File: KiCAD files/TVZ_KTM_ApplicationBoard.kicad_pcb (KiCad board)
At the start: 2 copper layers, 146 x 55 mm, 114 parts, among them J1 Conn_02x19_Odd_Even, J2 Conn_02x19_Odd_Even, J3 Conn_02x19_Odd_Even, J4 Conn_02x19_Odd_Even, SW1 EG1271A, SW2 EG1271A, SW3 EG1271A, SW4 EG1271A, U1 LM75B, U2 MCP2551-I-P, U3 MCP2551-I-P

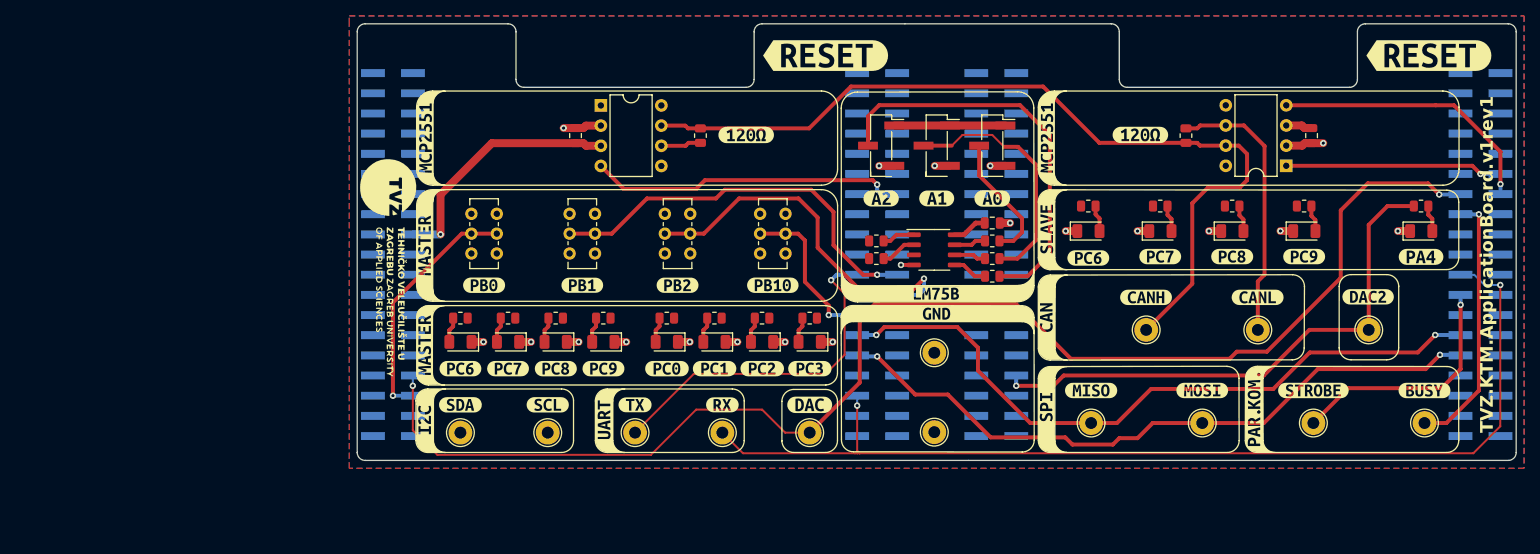
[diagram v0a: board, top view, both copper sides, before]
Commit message: update
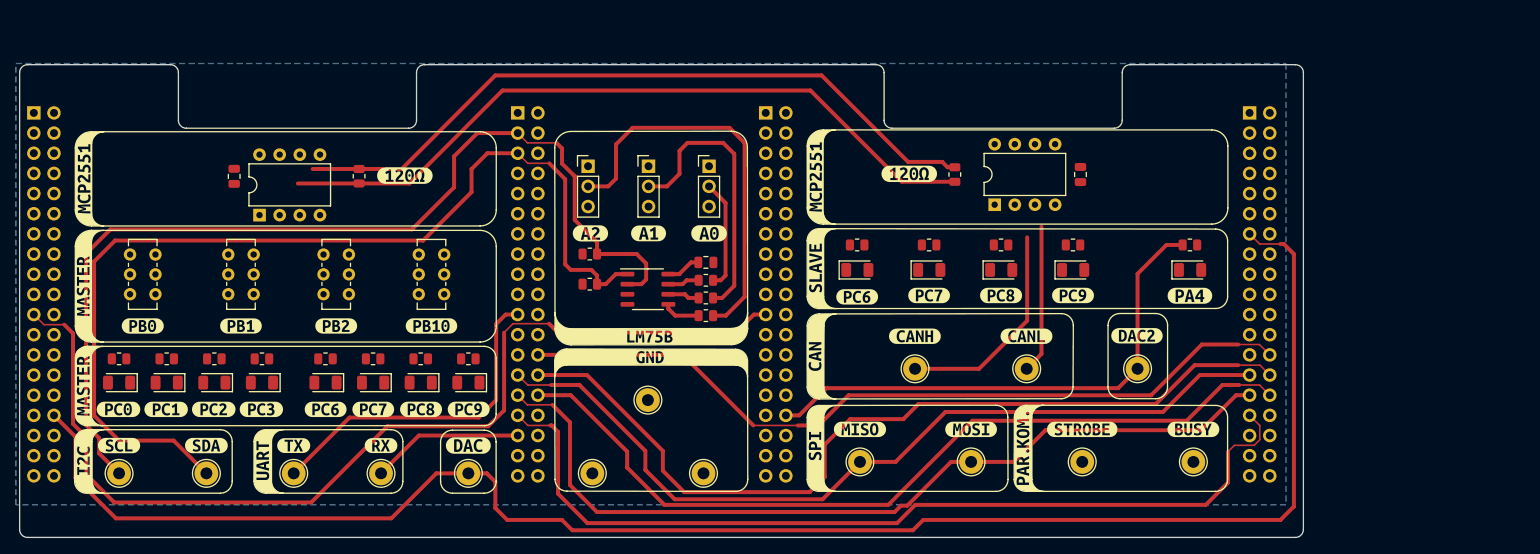
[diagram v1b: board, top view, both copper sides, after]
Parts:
- removed G***: LOGO, Footprint:tvz3
- removed kibuzzard-63D0F0B6 (x2): G***, kibuzzard-63D0F0B6
- added TP15: TestPoint, Footprint:KEYS4952, F.Cu at (143.6, 106.6)
- J1, J2, J3, J4: footprint Connector_PinSocket_2.54mm:PinSocket_2x19_P2.54mm_Vertical_SMD -> Connector_PinSocket_2.54mm:PinSocket_2x19_P2.54mm_Vertical
- JP1, JP4, JP5: footprint Connector_PinHeader_2.54mm:PinHeader_1x03_P2.54mm_Vertical_SMD_Pin1Right -> Connector_PinHeader_2.54mm:PinHeader_1x03_P2.54mm_Vertical
- moved kibuzzard-64A69B51 69.3 mm to (69.9, 98.6)
- moved kibuzzard-64A69B71 69.3 mm to (75.9, 98.6)
- moved kibuzzard-64A69B81 69.3 mm to (81.9, 98.6)
- moved kibuzzard-64A69B8B 69.3 mm to (87.9, 98.6)
- moved TP6 54.2 mm to (70.0, 106.6)
- moved kibuzzard-63D0FB98 54.2 mm to (70.0, 103.1)
- moved J2 48.7 mm to (120.2, 61.2)
- moved J1 48.6 mm to (59.3, 61.2)
- moved U2 45.2 mm to (87.7, 74.1), turned to 90 degrees
- moved TP9 43.4 mm to (129.6, 106.6)
- moved C2 43.3 mm to (84.5, 69.2)
- moved D10 43.3 mm to (76.0, 95.2)
- moved D11 43.3 mm to (82.0, 95.2)
- moved D12 43.3 mm to (88.0, 95.2)
- moved D5 43.3 mm to (96.0, 95.2)
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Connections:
- R10 pad 1: PC0_1 -> PC6_1
- R11 pad 1: PC1_1 -> PC7_1
- R12 pad 1: PC2_1 -> PC8_1
- R13 pad 1: PC3_1 -> PC9_1
- R14 pad 1: PC6_1 -> PC0_1
- R15 pad 1: PC7_1 -> PC1_1
- R16 pad 1: PC8_1 -> PC2_1
- R17 pad 1: PC9_1 -> PC3_1
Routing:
- net PB7_1: track 0.00 -> 127.9 mm
- net PB9_1: track 4.14 -> 125.4 mm
- net PB8_1: track 4.53 -> 125.1 mm
- net PB3_SCK: track 0.00 -> 113.9 mm
- net PA10_1: track 132.0 -> 19.2 mm, vias 2 -> 0
- net PB14_1: track 0.00 -> 109.3 mm
- net PB13_1: track 0.00 -> 105.9 mm
- net PB15_1: track 0.00 -> 100.6 mm
- net /CANL: track 39.7 -> 109.2 mm
- net PB2_1: track 50.5 -> 0.00 mm, vias 1 -> 0
- net PB1_1: track 47.1 -> 0.00 mm, vias 1 -> 0
- net PA11_1: track 40.1 -> 0.00 mm, vias 1 -> 0
- net PA4_1: track 172.8 -> 211.5 mm, vias 2 -> 0
- net GND: track 37.9 -> 0.00 mm, vias 20 -> 0
- net +5V: track 34.8 -> 0.00 mm, vias 1 -> 0
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- removed copper zone on F.Cu, net GND
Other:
- board size 146 x 55 mm -> 161.7 x 59.5 mm
- board text removed: "TVZ.KTM.ApplicationBoard.v1rev1"
